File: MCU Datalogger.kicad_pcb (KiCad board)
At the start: 2 copper layers, 29 parts, among them J1 Conn_01x04_Pin, J2 Conn_01x04_Pin, J3 Conn_01x09_Pin, J4 Conn_02x03_Odd_Even, U1 24LC1025, U2 DS1337S_, U3 24LC1025, U4 ATMEGA328P-AU, Y1 32.768 KHZ, Y2 16 MHZ

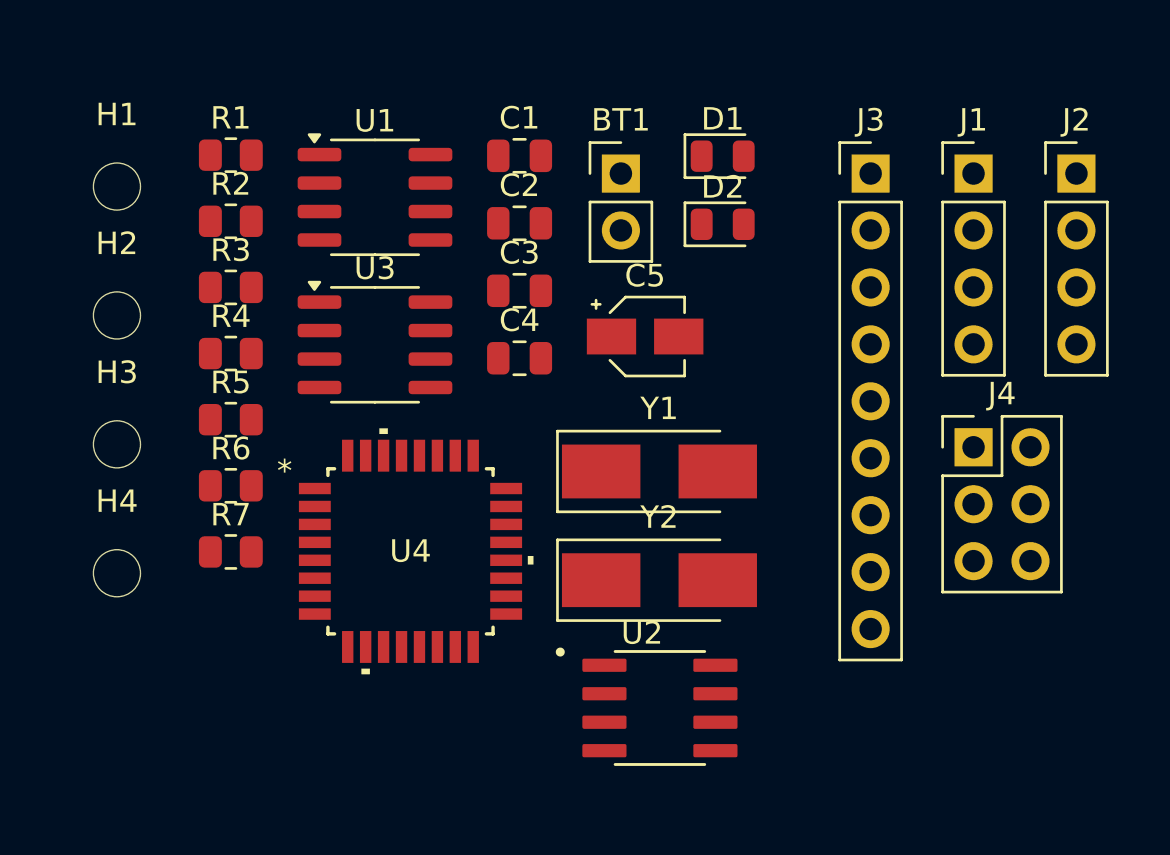
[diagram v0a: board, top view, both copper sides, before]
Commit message: placed components
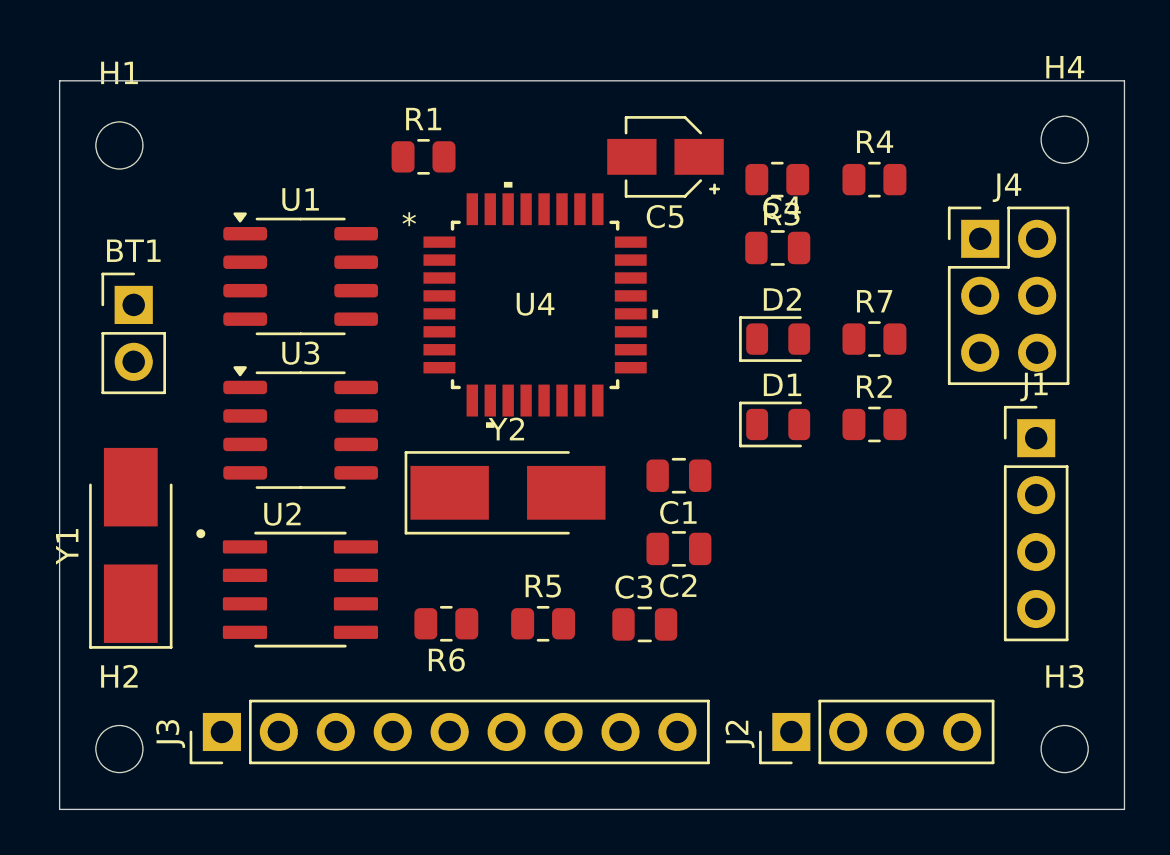
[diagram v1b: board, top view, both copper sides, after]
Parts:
- moved H4 46.5 mm to (179.8, 87.6)
- moved H3 44.4 mm to (179.8, 114.8)
- moved J3 38.2 mm to (142.2, 114.0), turned to 90 degrees
- moved R7 30.2 mm to (171.3, 96.5)
- moved R2 30.1 mm to (171.3, 100.3)
- moved R4 29.7 mm to (171.3, 89.4)
- moved J2 28.0 mm to (167.6, 114.0), turned to 90 degrees
- moved R3 24.8 mm to (167.0, 89.4), turned to 180 degrees
- moved Y1 23.8 mm to (138.2, 105.7), turned to 90 degrees
- moved BT1 22.5 mm to (138.3, 95.0)
- moved H2 19.3 mm to (137.7, 114.8)
- moved U2 16.9 mm to (145.7, 107.7)
- moved R5 16.6 mm to (156.6, 109.2)
- moved C2 16.2 mm to (162.6, 105.9), turned to 180 degrees
- moved C1 15.9 mm to (162.6, 102.6), turned to 180 degrees
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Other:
- board outline added: 47.5 x 32.5 mm
